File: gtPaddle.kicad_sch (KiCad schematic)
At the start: 24 parts, among them IC1 74157N, IC2 74157N, J1 Conn_01x02_Pin, J2 Conn_01x02_Pin, J3 Conn_01x02_Pin, J4 Conn_01x02_Pin, Q1 2N3904, U1 ADC0804LCN

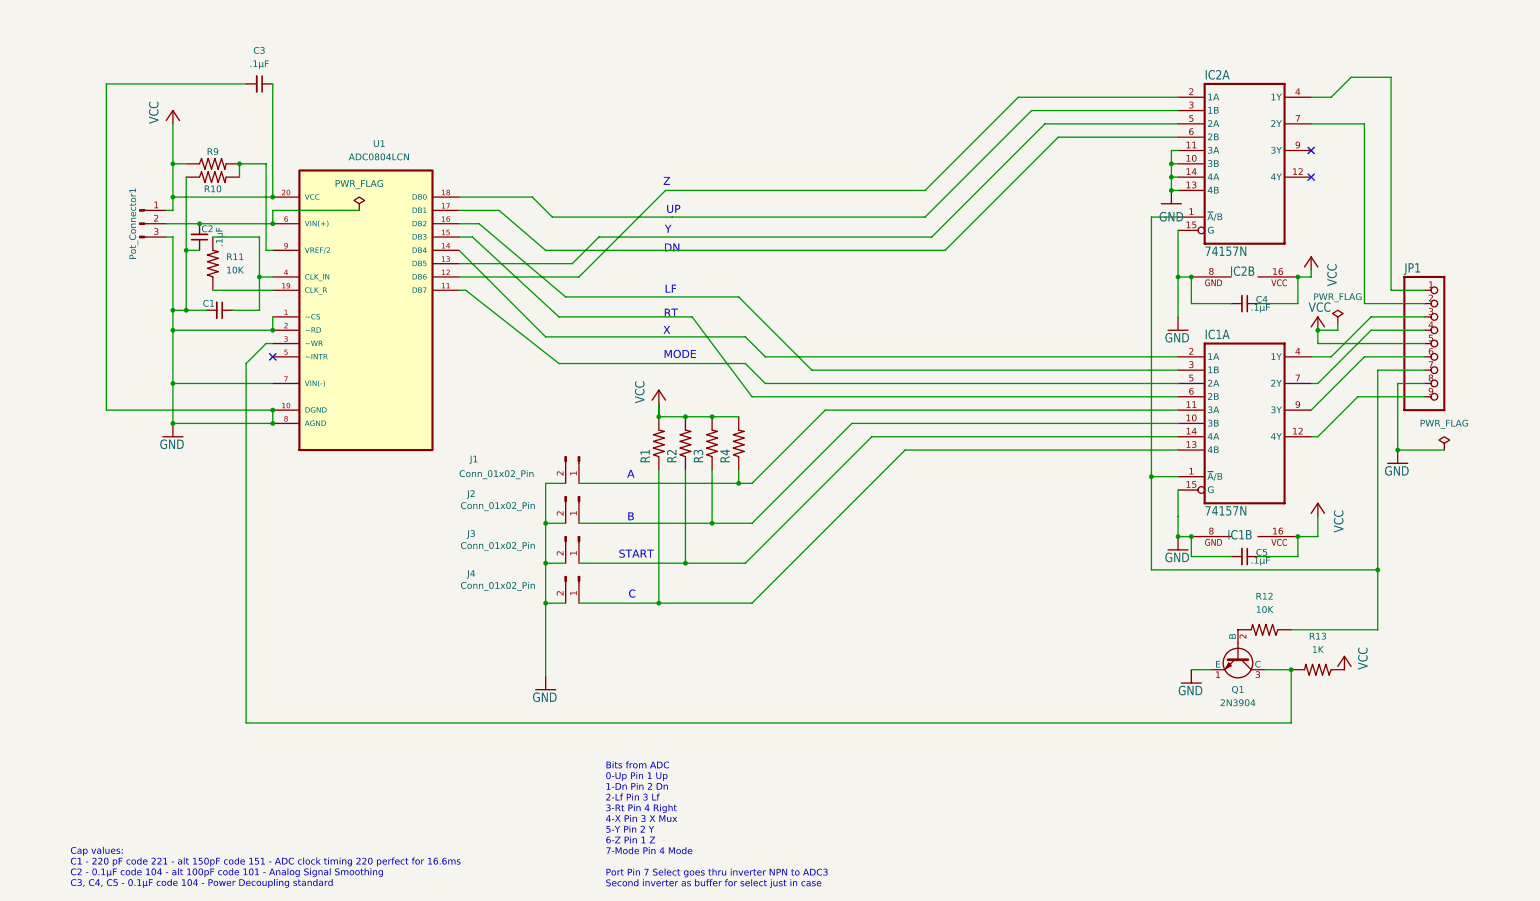
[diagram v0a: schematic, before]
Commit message: Individual headers first pass
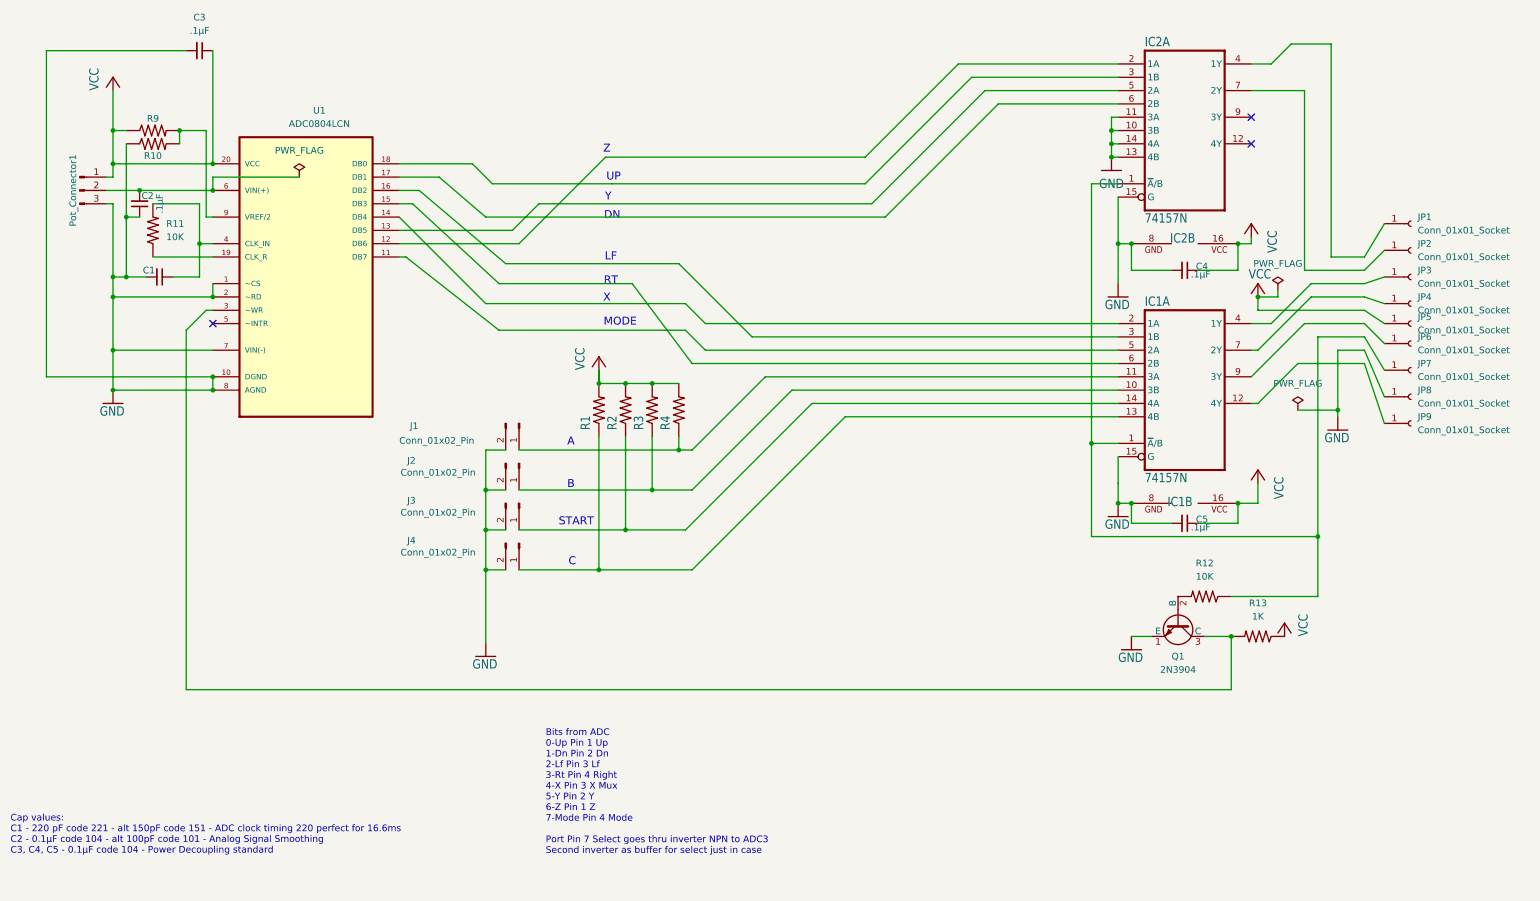
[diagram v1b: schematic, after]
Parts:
- removed JP1: PINHD-1X9, gpad1:1X09, symbol gpad1-eagle-import:PINHD-1X9
- added JP1, JP2, JP3, JP4, JP5, JP6, JP7, JP8, JP9: Conn_01x01_Socket, Connector_Wire:SolderWire-0.75sqmm_1x01_D1.25mm_OD2.3mm, symbol Connector:Conn_01x01_Socket
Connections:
- net GND: now also JP8.1 (Pin_1)
- net VCC: now also JP5.1 (Pin_1)
- net at IC1.1 (~{A}/B), IC2.1 (~{A}/B), R12.1: now also JP7.1 (Pin_1)
- net at IC2.4 (1Y): now also JP1.1 (Pin_1)
- net at IC2.7 (2Y): now also JP2.1 (Pin_1)
- net at IC1.4 (1Y): now also JP3.1 (Pin_1)
- net at IC1.7 (2Y): now also JP4.1 (Pin_1)
- net at IC1.9 (3Y): now also JP6.1 (Pin_1)
- net at IC1.12 (4Y): now also JP9.1 (Pin_1)
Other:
- moved on the sheet: C1, C2, C3, C4, C5, IC1A, IC1B, IC2A, IC2B, J1, J2, J3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
